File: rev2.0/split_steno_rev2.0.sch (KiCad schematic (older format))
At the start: 65 parts, among them J1 Audio-Jack-4, SW1 SW_Push, U1 ATXMEGA128A4U-AU

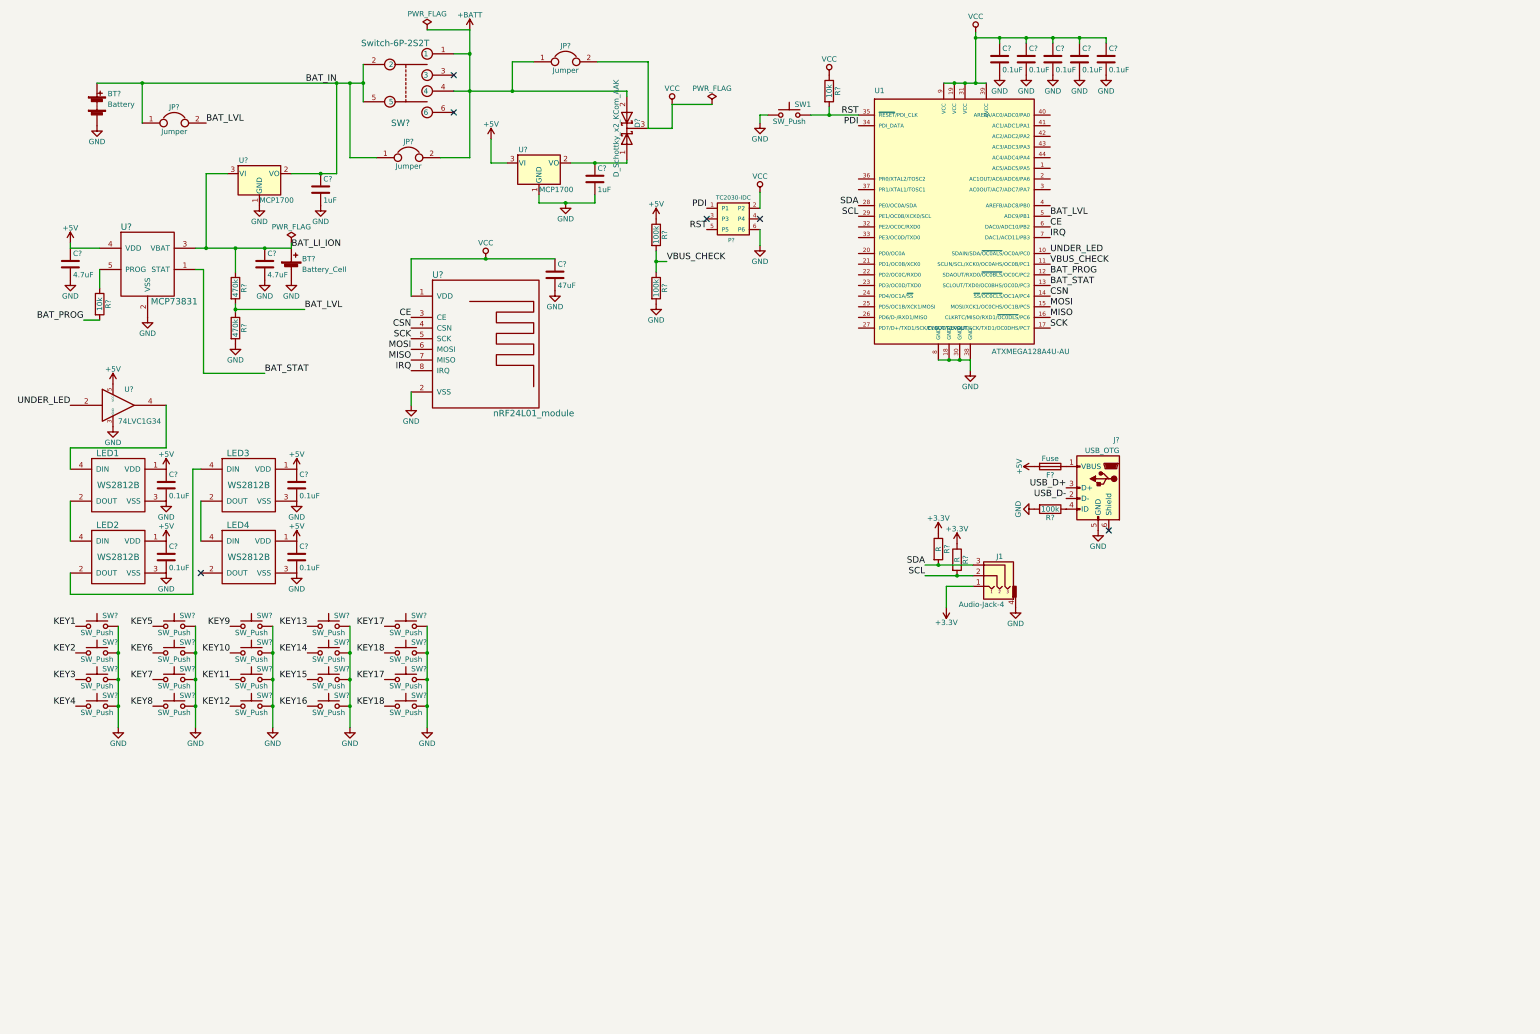
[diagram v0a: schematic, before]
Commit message: things
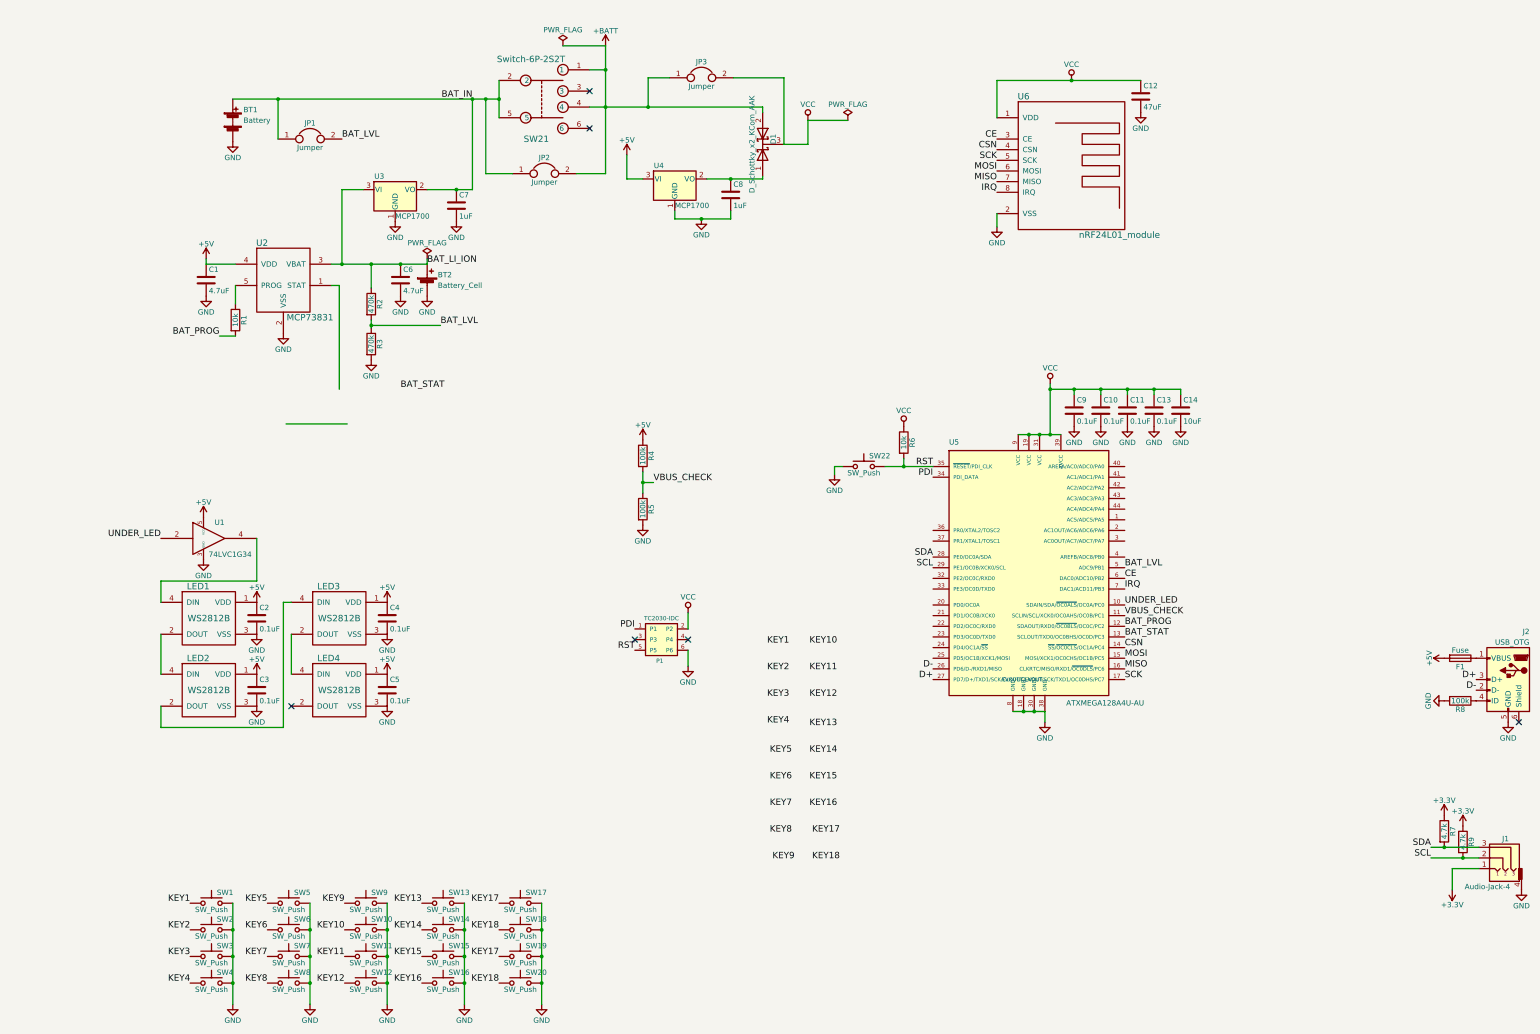
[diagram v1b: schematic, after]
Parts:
- C14: renamed from C?; value 0.1uF -> 10uF
- R7, R9: renamed from R?; value R -> 4.7k
- gave numbers to parts that had none: 55
- renumbered SW1 to SW22, U1 to U5
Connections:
- net labels added: D+, D-
- net labels removed: USB_D+, USB_D-
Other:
- moved on the sheet: BT1, BT2, C1, C10, C11, C12, C13, C14, C2, C3, C4, C5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
